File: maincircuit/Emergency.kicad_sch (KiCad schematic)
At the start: 10 parts, among them J5 Conn_01x02_Pin, Q1 Q_NMOS, Q2 Q_NMOS, U1 TLP152

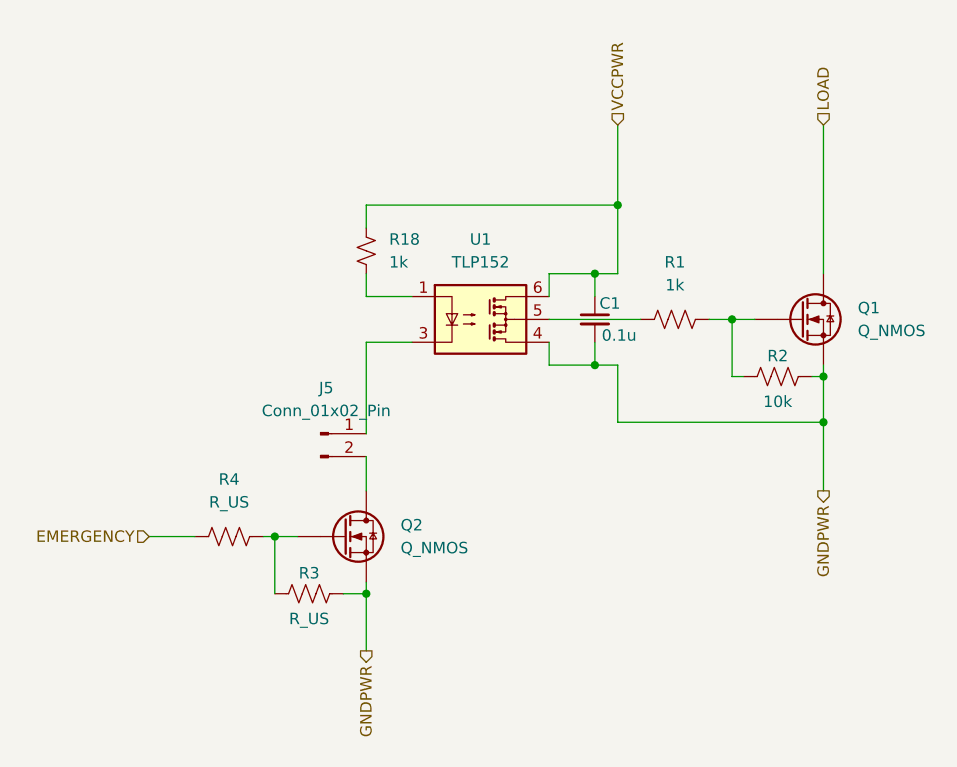
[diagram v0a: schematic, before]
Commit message: [add]ControlCircuit完成
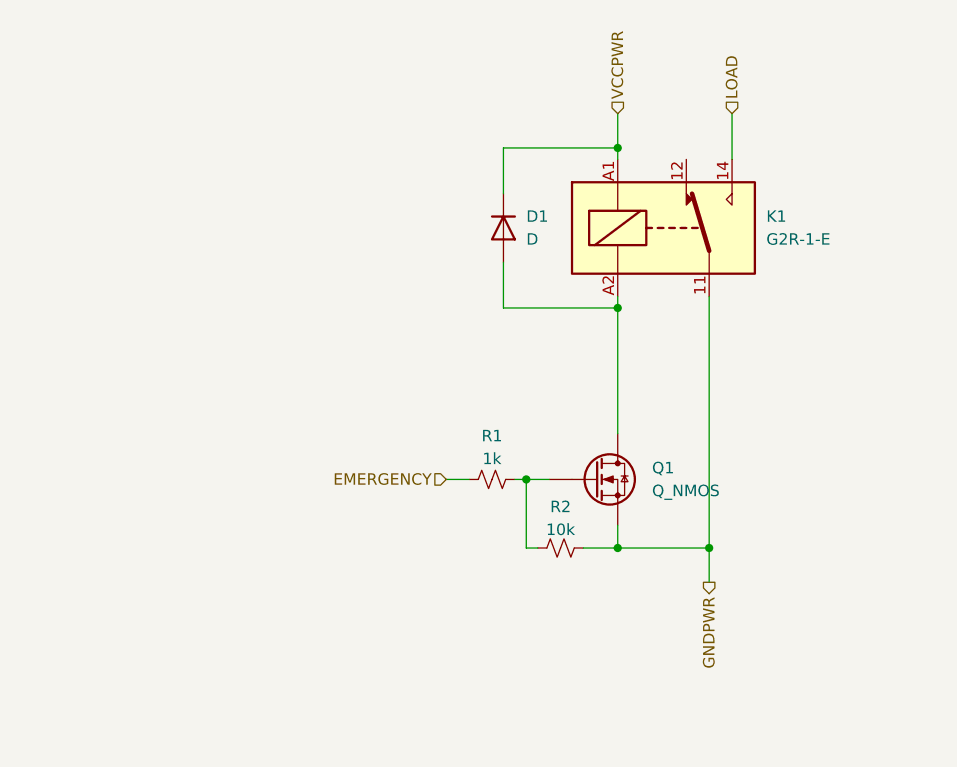
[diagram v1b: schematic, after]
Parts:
- removed C1: 0.1u, Capacitor_SMD:C_0603_1608Metric_Pad1.08x0.95mm_HandSolder, symbol Device:C_Small
- removed J5: Conn_01x02_Pin, symbol Connector:Conn_01x02_Pin
- removed Q2: Q_NMOS, symbol Device:Q_NMOS
- removed R1: 1k, symbol Device:R_US
- removed R18: 1k, symbol Device:R_Small_US
- removed R2: 10k, symbol Device:R_US
- removed R3, R4: R_US, symbol Device:R_US
- removed U1: TLP152, Package_SO:SO-5-6_4.55x3.7mm_P1.27mm, symbol Library:TLP152
- added D1: D, symbol Device:D
- added K1: G2R-1-E, Library:G2R-1-E, symbol Library:G2R-1-E
- added R1: 1k, symbol Device:R_Small_US
- added R2: 10k, symbol Device:R_Small_US
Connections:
- net EMERGENCY: now also R1.1
- net GNDPWR: now also K1.11, R2.2
- net LOAD: now also K1.14; no longer Q1.D
- net VCCPWR: now also D1.1 (K), K1.A1
- net at Q1.G: now also R1.2, R2.1
- new net: D1.2 (A), K1.A2, Q1.D
